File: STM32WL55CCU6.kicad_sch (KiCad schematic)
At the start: 25 parts, among them J6 BOOT0_Jumper, SW3 Switch_NX3L1T3157GMZ, U4 STM32WL55CCU6

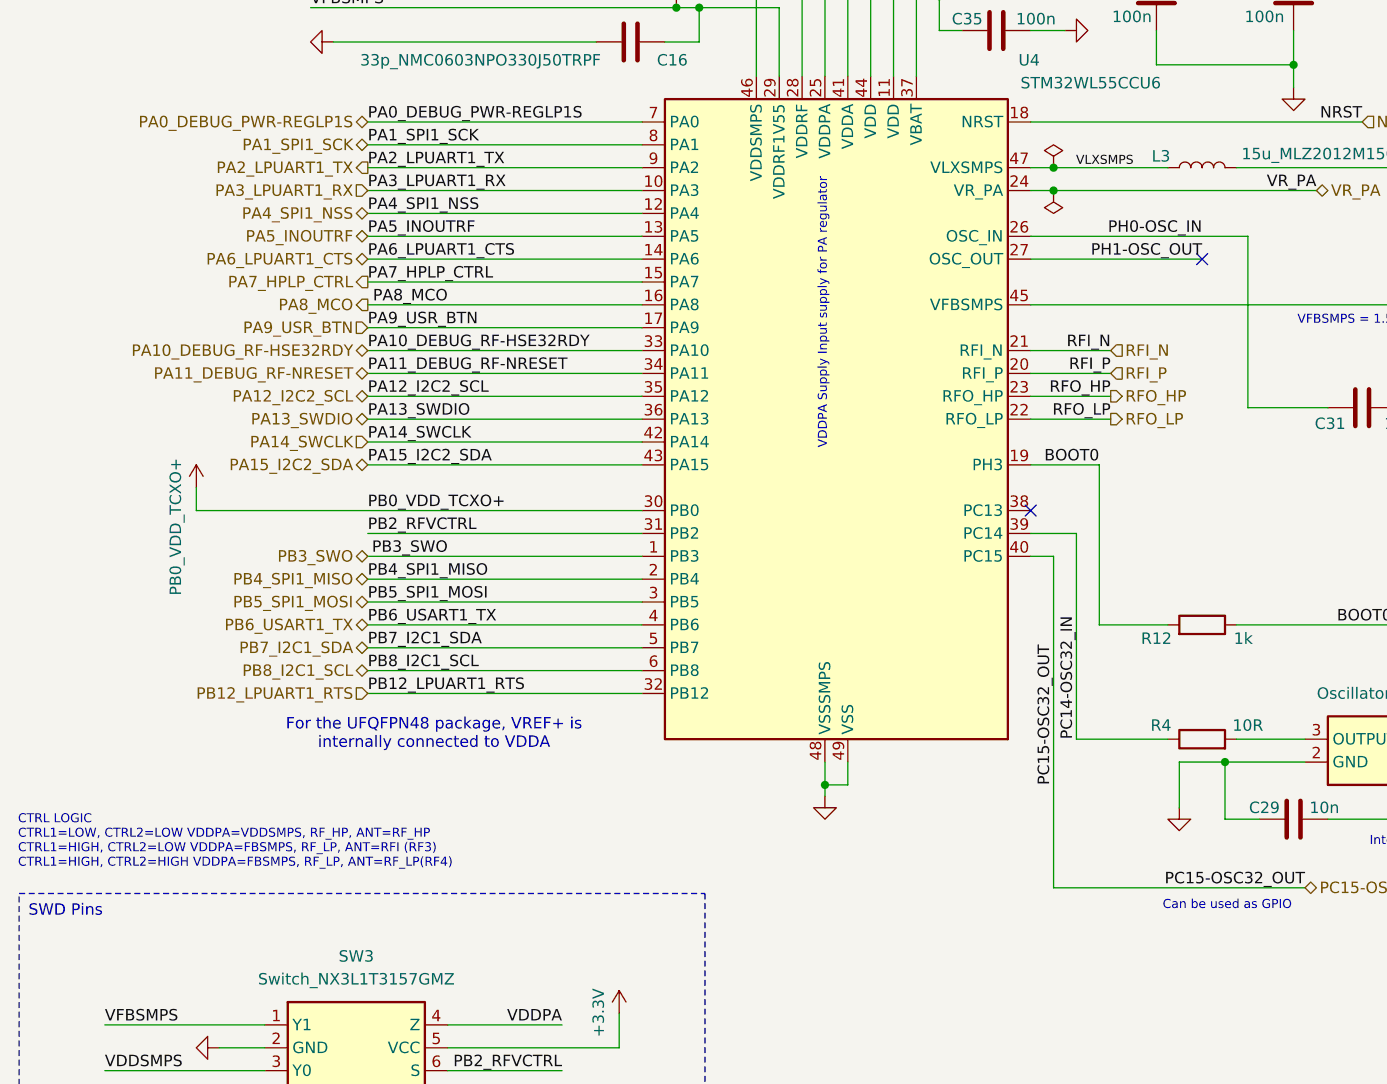
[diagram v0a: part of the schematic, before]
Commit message: Update
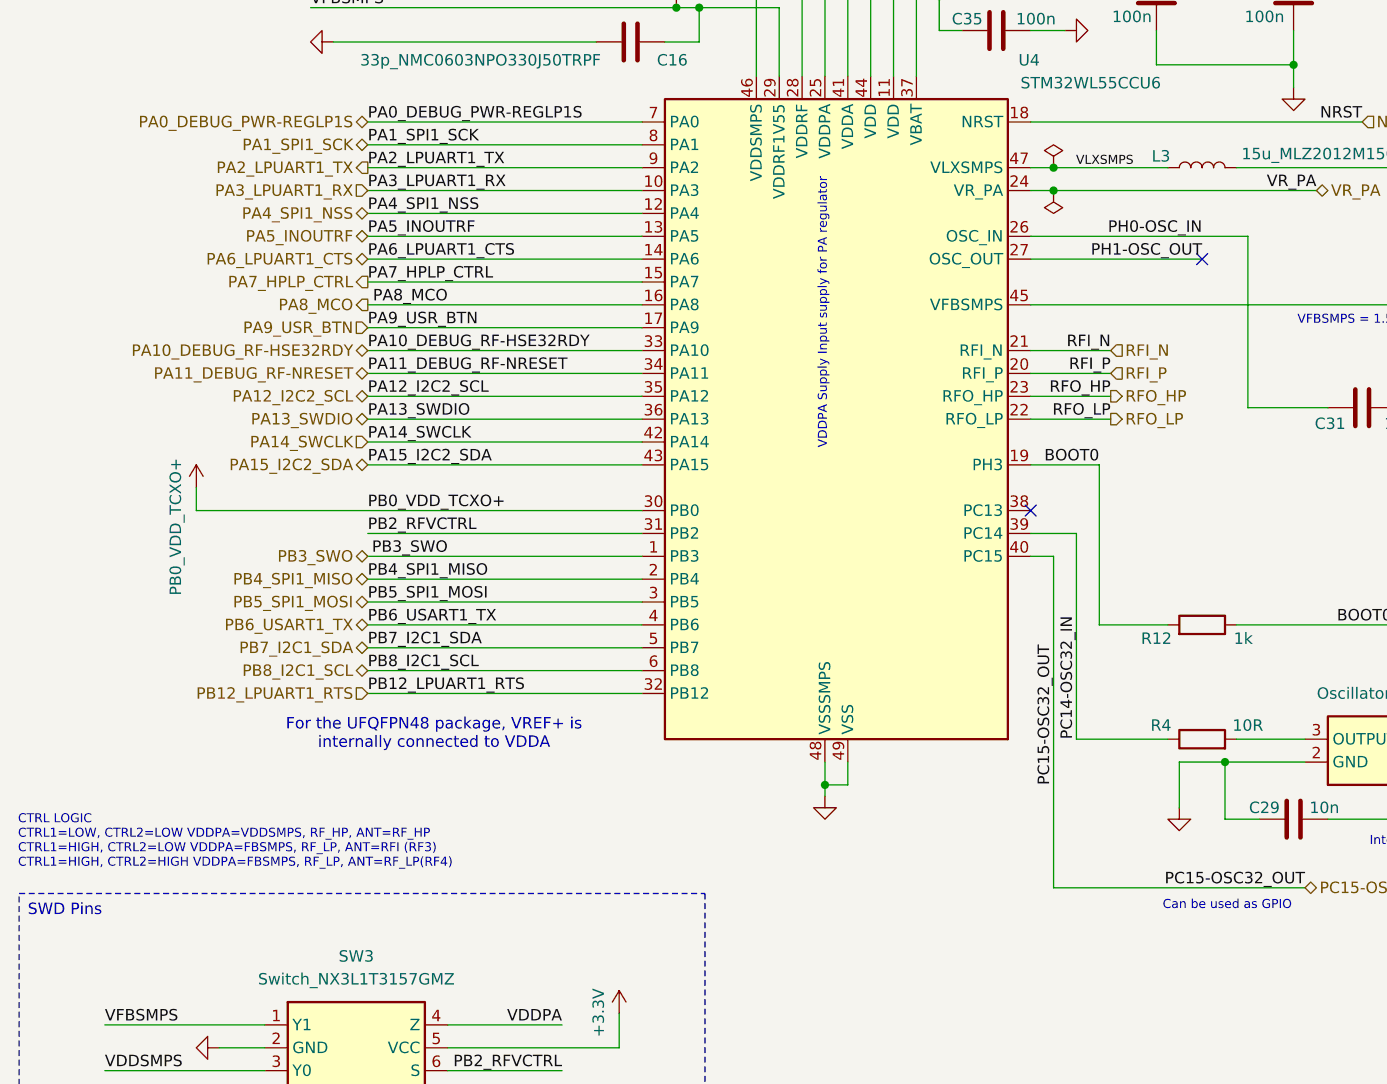
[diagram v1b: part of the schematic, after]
